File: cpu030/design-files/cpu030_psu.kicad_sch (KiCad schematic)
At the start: 2 parts, among them J901 ATX-24

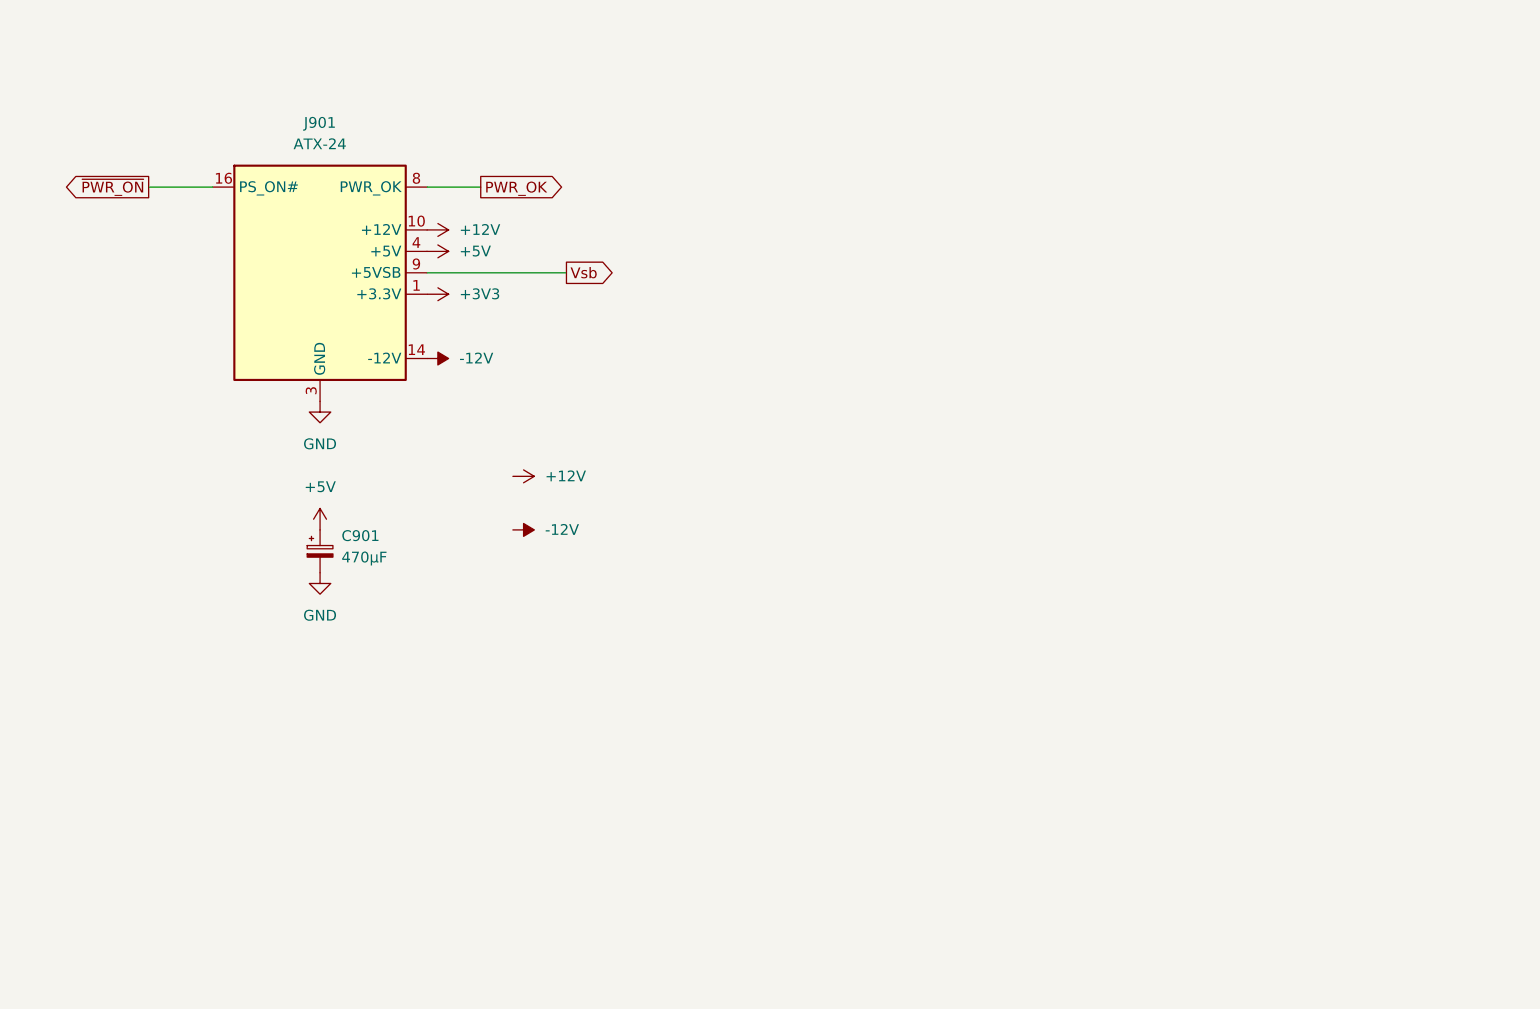
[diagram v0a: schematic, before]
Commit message: Add ATtiny85 as a PSU controller.
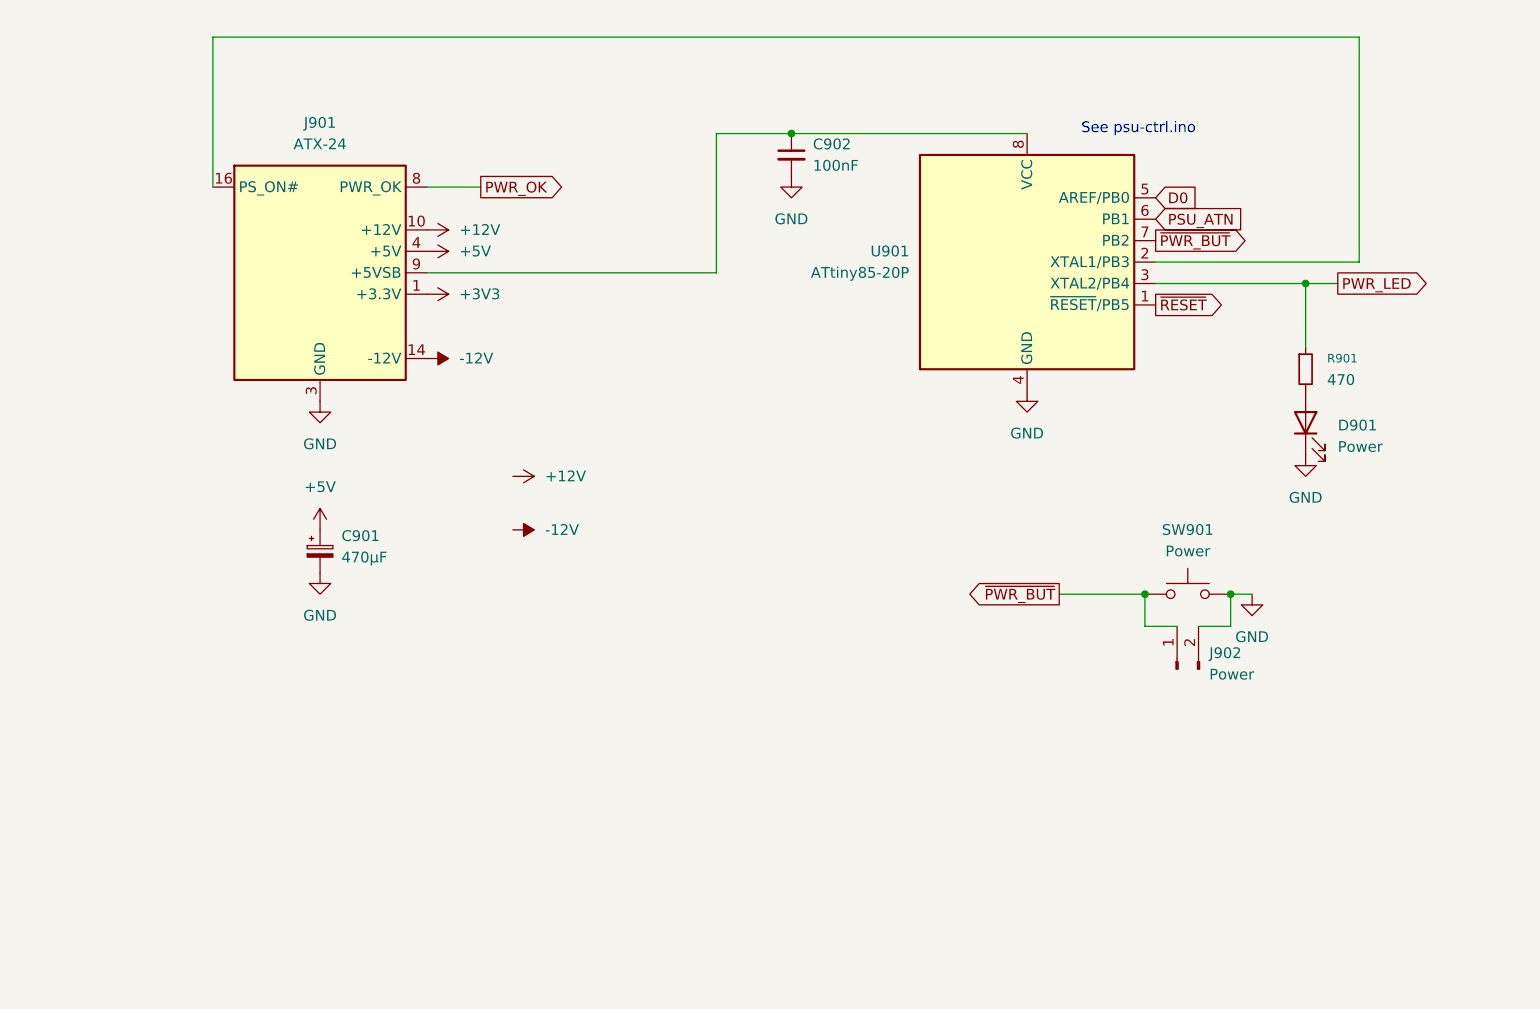
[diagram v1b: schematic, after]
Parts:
- added C902: 100nF, Capacitor_SMD:C_0805_2012Metric, symbol Device:C_Small
- added D901: Power, LED_THT:LED_D3.0mm, symbol Device:LED
- added J902: Power, Connector_PinHeader_2.54mm:PinHeader_1x02_P2.54mm_Vertical, symbol Connector:Conn_01x02_Pin
- added R901: 470, Resistor_SMD:R_0805_2012Metric, symbol Device:R_Small
- added SW901: Power, Button_Switch_THT:SW_PUSH_6mm, symbol Switch:SW_Push
- added U901: ATtiny85-20P, Package_DIP:DIP-8_W7.62mm_Socket, symbol MCU_Microchip_ATtiny:ATtiny85-20P
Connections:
- net GND: now also C902.2, D901.1 (K), J902.2 (Pin_2), SW901.2, U901.4 (GND)
- net Vsb: no longer names the net of J901.9 (+5VSB)
- net Vsb: now also C902.1, U901.8 (VCC)
- net ~{PWR_ON}: no longer names the net of J901.16 (PS_ON#)
- net ~{PWR_ON}: now also U901.2 (XTAL1/PB3)
- new net: D901.2 (A), R901.2
- new net D0: U901.5 (AREF/PB0)
- new net PSU_ATN: U901.6 (PB1)
- new net PWR_LED: R901.1, U901.3 (XTAL2/PB4)
- new net ~{PWR_BUT}: J902.1 (Pin_1), SW901.1, U901.7 (PB2)
- new net ~{RESET}: U901.1 (~{RESET}/PB5)
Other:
- note added: "See psu-ctrl.ino"

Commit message: Checkpoint -- I'm going to re-arrange the board a bit and make it 6 layers, putting CPU address and data busses on their own internal signal layers.  Hopefully this detangles the mess a bit.
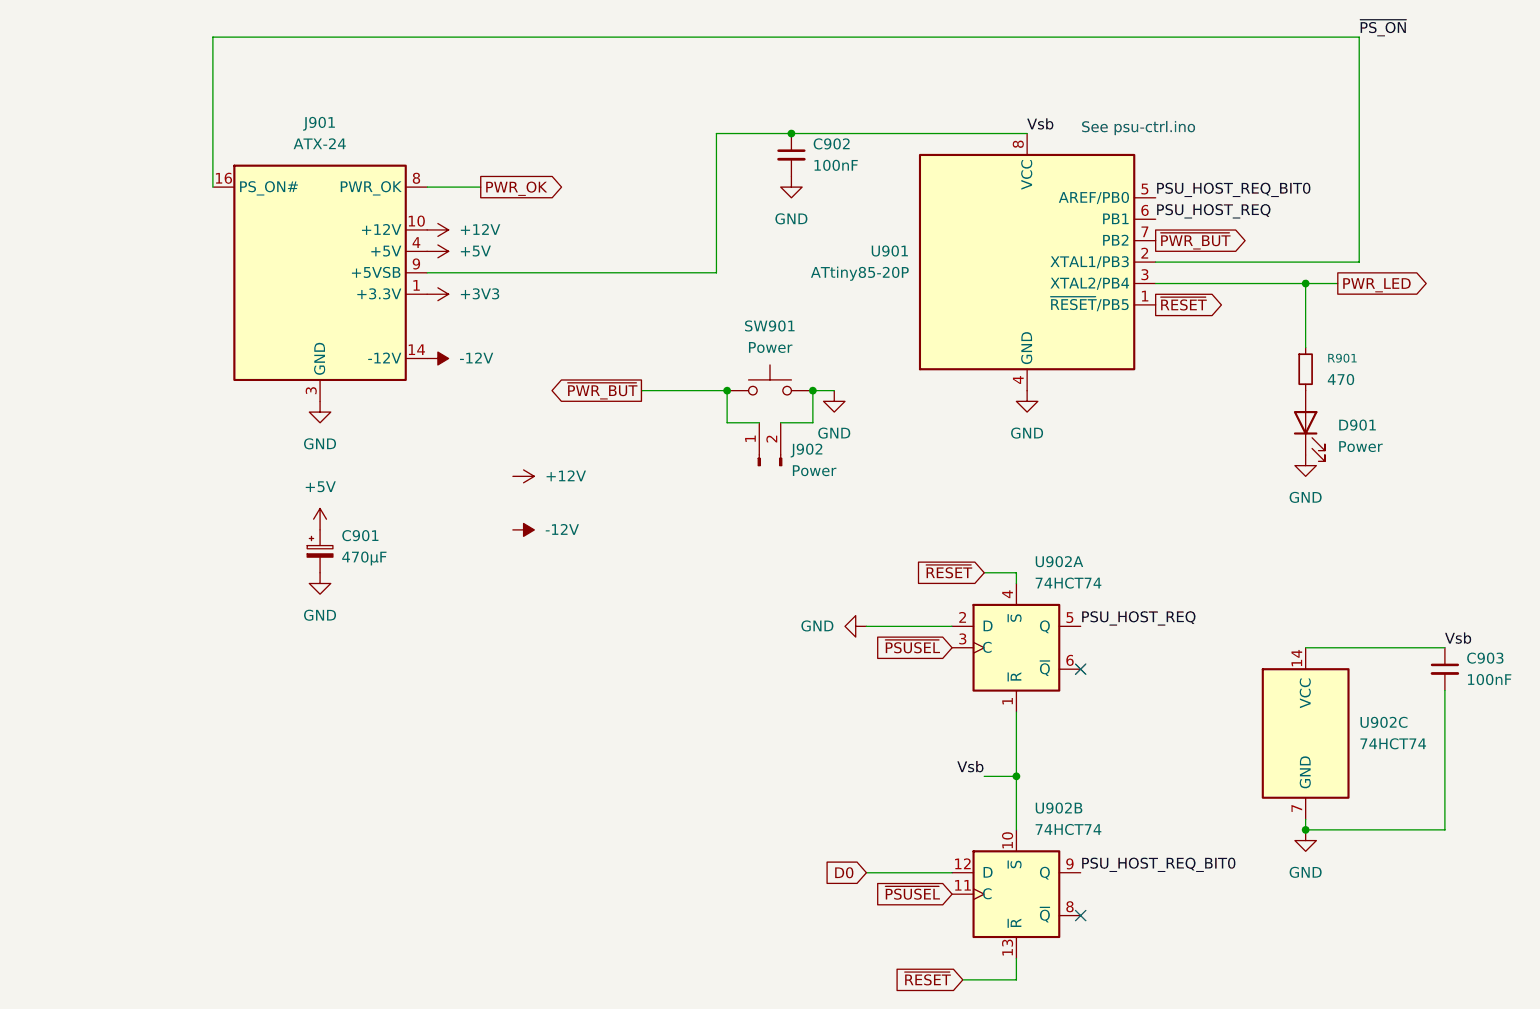
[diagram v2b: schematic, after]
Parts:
- added C903: 100nF, Capacitor_SMD:C_0805_2012Metric, symbol Device:C_Small
- added U902: 74HCT74, Package_SO:SOIC-14_3.9x8.7mm_P1.27mm, symbol 74xx:74HC74
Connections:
- net D0: now also U902.12 (D); no longer U901.5 (AREF/PB0)
- net GND: now also C903.2, U902.2 (D), U902.7 (GND)
- net ~{RESET}: now also U902.13 (~{R}), U902.4 (~{S})
- net Vsb: now reaches C902.1, J901.9 (+5VSB), U901.8 (VCC)
- net Vsb: now also C903.1, U902.1 (~{R}), U902.10 (~{S}), U902.14 (VCC)
- net ~{PS_ON}: now reaches J901.16 (PS_ON#), U901.2 (XTAL1/PB3)
- net PSU_ATN renamed PSU_HOST_REQ
- net PSU_HOST_REQ: now also U902.5 (Q)
- new net PSU_HOST_REQ_BIT0: U901.5 (AREF/PB0), U902.9 (Q)
- new net ~{PSUSEL}: U902.11 (C), U902.3 (C)
- no-connect marks 0 -> 2
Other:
- moved on the sheet: J902, SW901
